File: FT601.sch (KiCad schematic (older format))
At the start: 23 parts, among them U1 FT601, U2 ESD7016, U4 ECP5, U5 Si5351, X1 GSB443133HR, Y1 FL3000027, Y2 ABM11-141-26.000MHZ

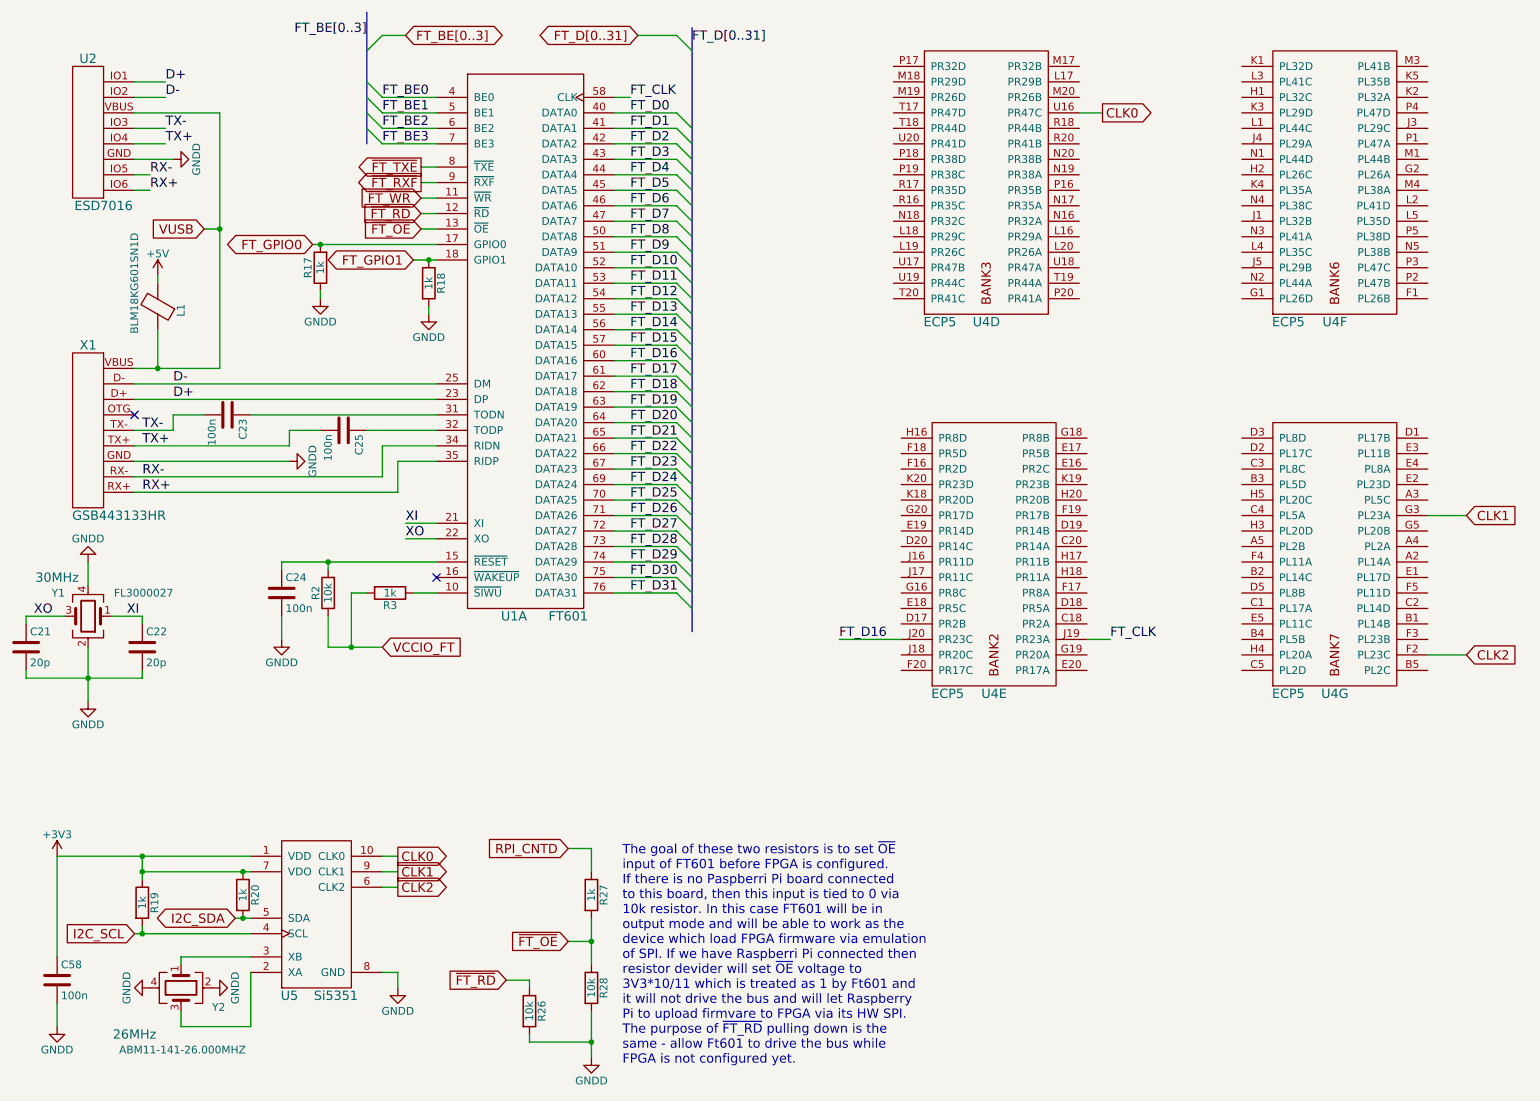
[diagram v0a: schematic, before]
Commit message: Right before Sitch power retracing
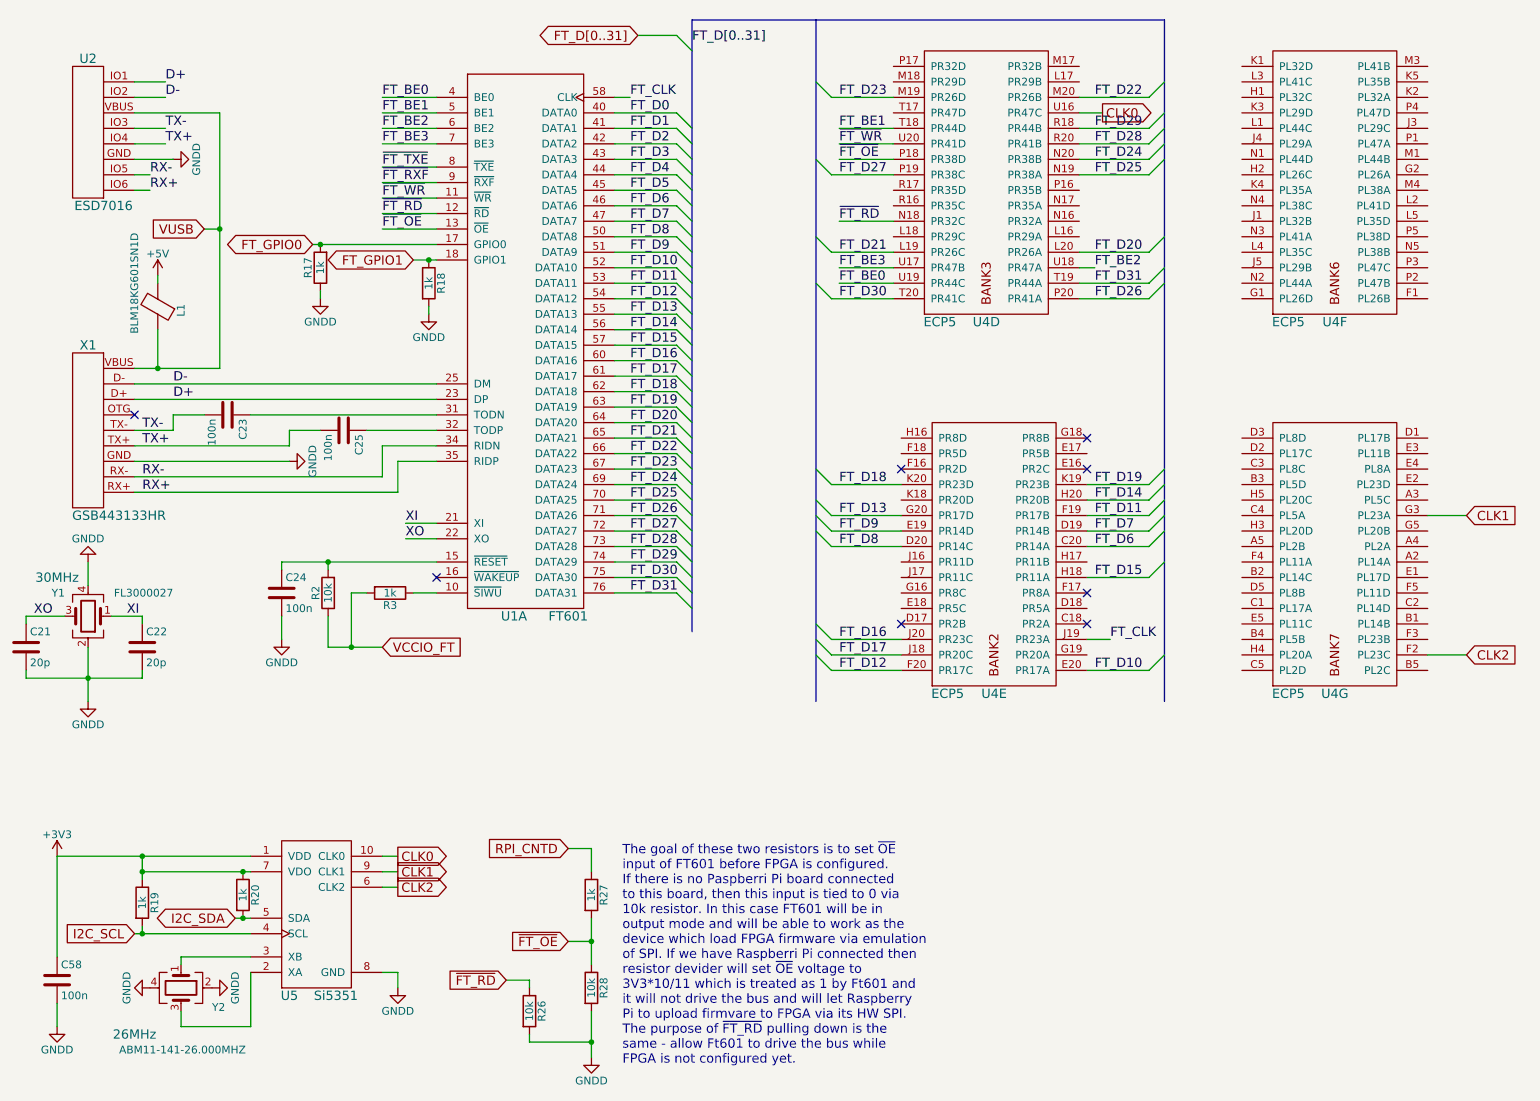
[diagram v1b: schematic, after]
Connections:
- net FT_BE0: now also U4.U19 (PR44C)
- net FT_BE1: now also U4.T18 (PR44D)
- net FT_BE2: now also U4.U18 (PR47A)
- net FT_BE3: now also U4.U17 (PR47B)
- net FT_D10: now also U4.E20 (PR17A)
- net FT_D11: now also U4.F19 (PR17B)
- net FT_D12: now also U4.F20 (PR17C)
- net FT_D13: now also U4.G20 (PR17D)
- net FT_D14: now also U4.H20 (PR20B)
- net FT_D15: now also U4.H18 (PR11A)
- net FT_D17: now also U4.J18 (PR20C)
- net FT_D18: now also U4.K20 (PR23D)
- net FT_D19: now also U4.K19 (PR23B)
- net FT_D20: now also U4.L20 (PR26A)
- net FT_D21: now also U4.L19 (PR26C)
- net FT_D22: now also U4.M20 (PR26B)
- net FT_D23: now also U4.M19 (PR26D)
- net FT_D24: now also U4.N20 (PR38B)
- net FT_D25: now also U4.N19 (PR38A)
- net FT_D26: now also U4.P20 (PR41A)
- net FT_D27: now also U4.P19 (PR38C)
- net FT_D28: now also U4.R20 (PR41B)
- net FT_D29: now also U4.R18 (PR44B)
- net FT_D30: now also U4.T20 (PR41C)
- net FT_D31: now also U4.T19 (PR44A)
- net FT_D6: now also U4.C20 (PR14A)
- net FT_D7: now also U4.D19 (PR14B)
- net FT_D8: now also U4.D20 (PR14C)
- net FT_D9: now also U4.E19 (PR14D)
- net ~FT_OE: now also U4.P18 (PR38D)
- net ~FT_RD: now also U4.N18 (PR32C)
- net ~FT_WR: now also U4.U20 (PR41D)
- no-connect marks 2 -> 8
